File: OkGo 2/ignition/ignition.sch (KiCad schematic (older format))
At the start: 30 parts, among them P101 CONN_01X02, P102 ANT, U101 TSR 0.5-2433, U102 SWD, U103 STM32F071CBT6, U104 RFM95W, Y101 8MHz

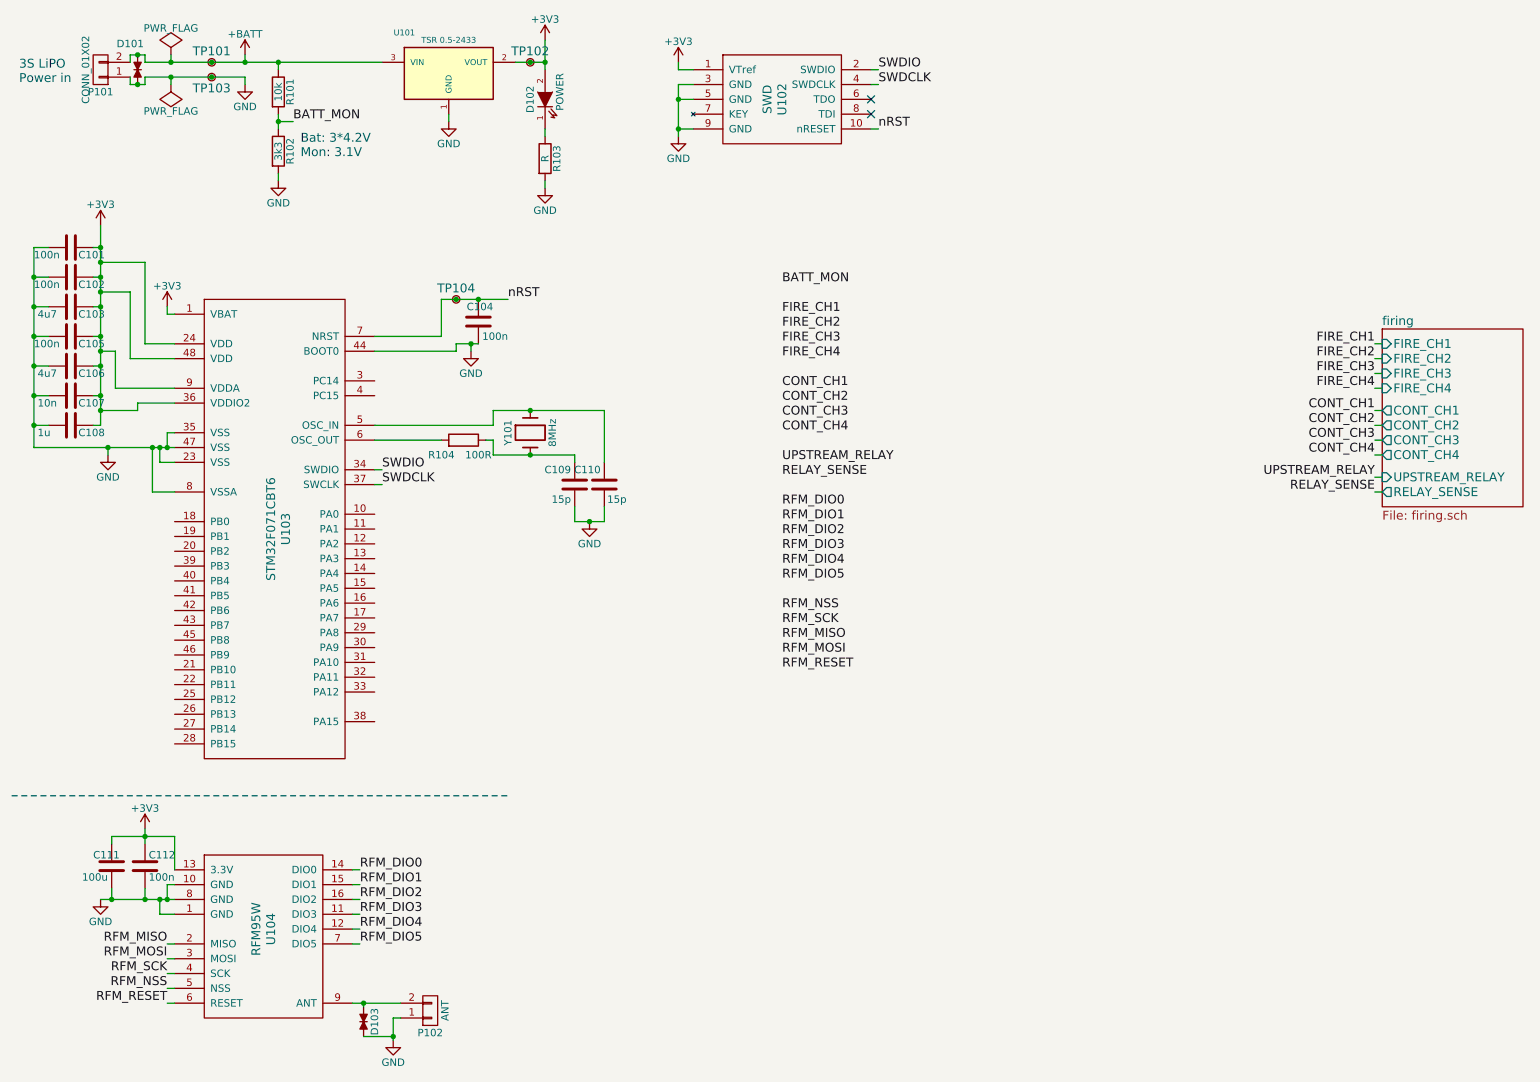
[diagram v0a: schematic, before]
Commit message: Lots and lots of part selections and small mods
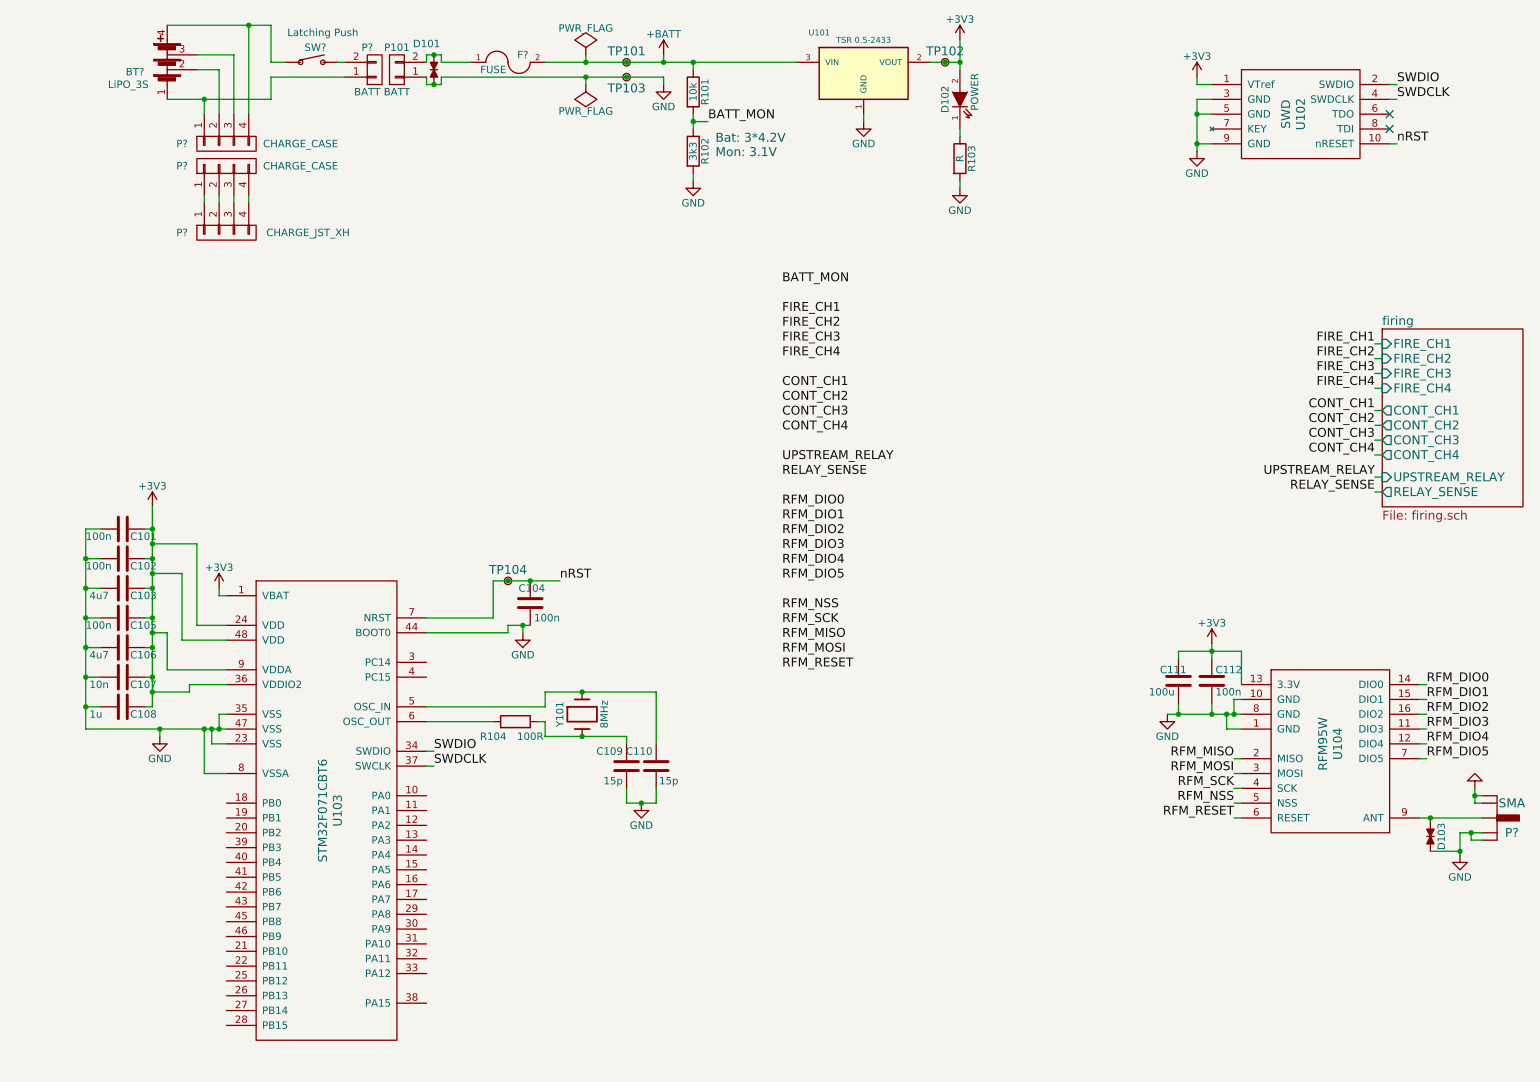
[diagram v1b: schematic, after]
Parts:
- removed P102: ANT, symbol CONN_01X02
- added BT?: LiPO_3S, symbol LiPO_3S
- added F?: FUSE, symbol FUSE
- added P?: SMA, common:SMA-142-0701-801, symbol SMA
- added P? (x2): CHARGE_CASE, symbol CONN_01X04
- added P?: BATT, symbol CONN_01X02
- added P?: CHARGE_JST_XH, symbol CONN_01X04
- added SW?: Latching Push, symbol SPST_small
- P101: value CONN_01X02 -> BATT
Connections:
- net +BATT: now also F?.2; no longer D101.1, P101.2 (P2)
- net GND: now also P?.2 (GND), P?.3 (GND), P?.4 (GND), P?.5 (GND)
- net at D103.1, U104.9 (ANT): now also P?.1 (RF)
- new net: D101.1, F?.1, P101.2 (P2)
- new net: BT?.1, P?.1 (P1), P?.1 (P1)
- new net: BT?.2, P?.2 (P2)
- new net: BT?.3, P?.3 (P3)
- new net: BT?.4, P?.4 (P4), SW?.1
- new net: P?.2 (P2), SW?.2
- new net: P?.1 (P1), P?.1 (P1)
- new net: P?.2 (P2), P?.2 (P2)
- new net: P?.3 (P3), P?.3 (P3)
- new net: P?.4 (P4), P?.4 (P4)
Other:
- note removed: "3S LiPO\nPower in"
- moved on the sheet: C101, C102, C103, C104, C105, C106, C107, C108, C109, C110, C111, C112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
